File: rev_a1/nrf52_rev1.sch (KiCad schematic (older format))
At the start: 27 parts, among them P1 CONN_01X18, P2 CONN_01X18, P3 USB_OTG, U1 nRF52832, U2 CP2102, U3 LT1129CST-3.3, Y1 32K, Y2 32M

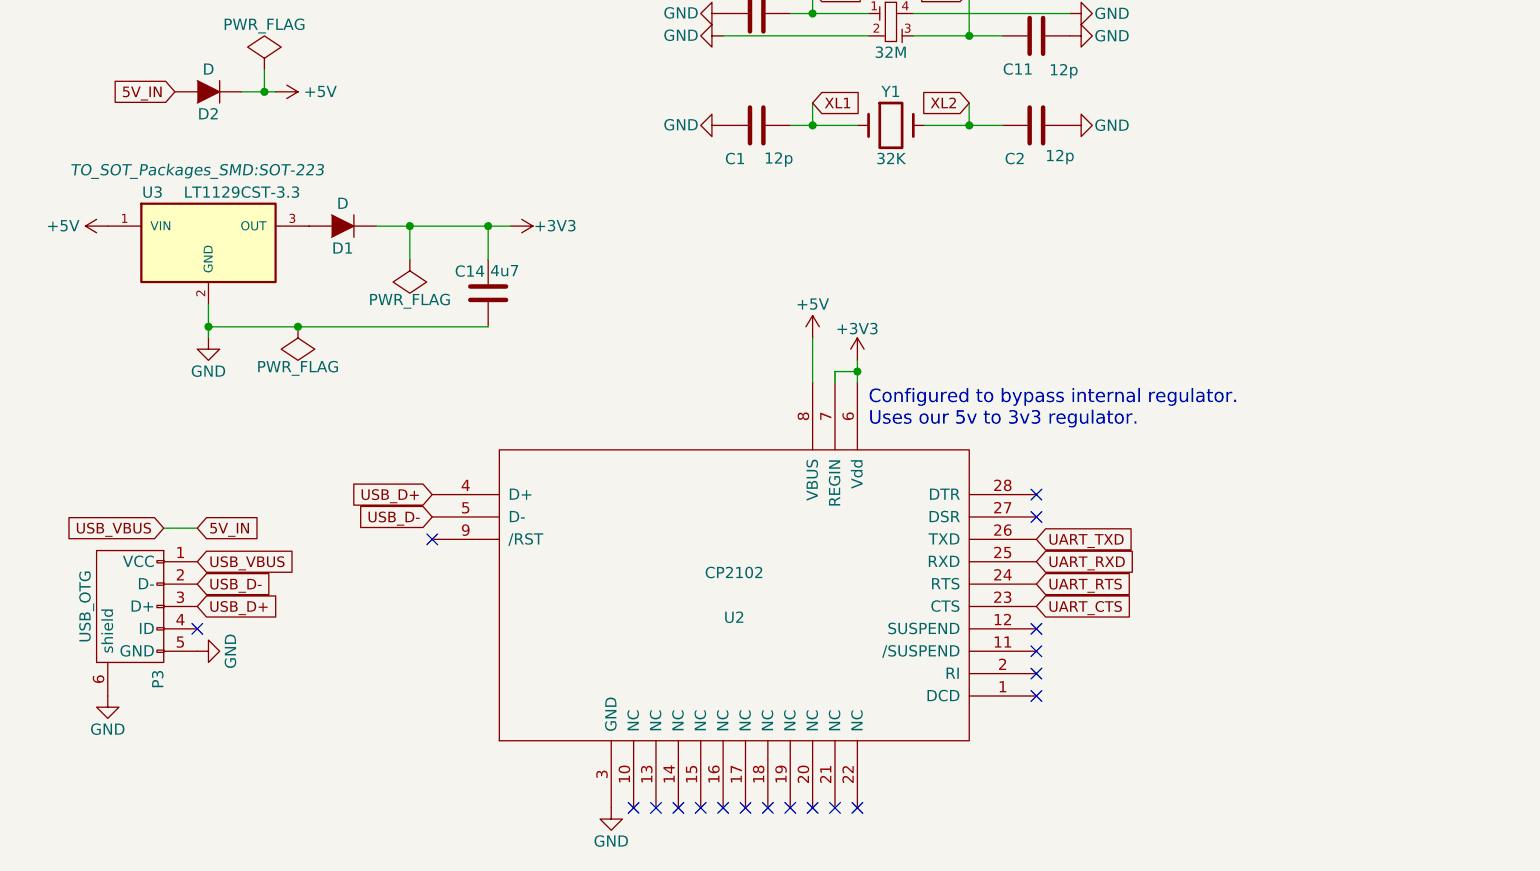
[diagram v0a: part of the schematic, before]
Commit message: wipwipwip
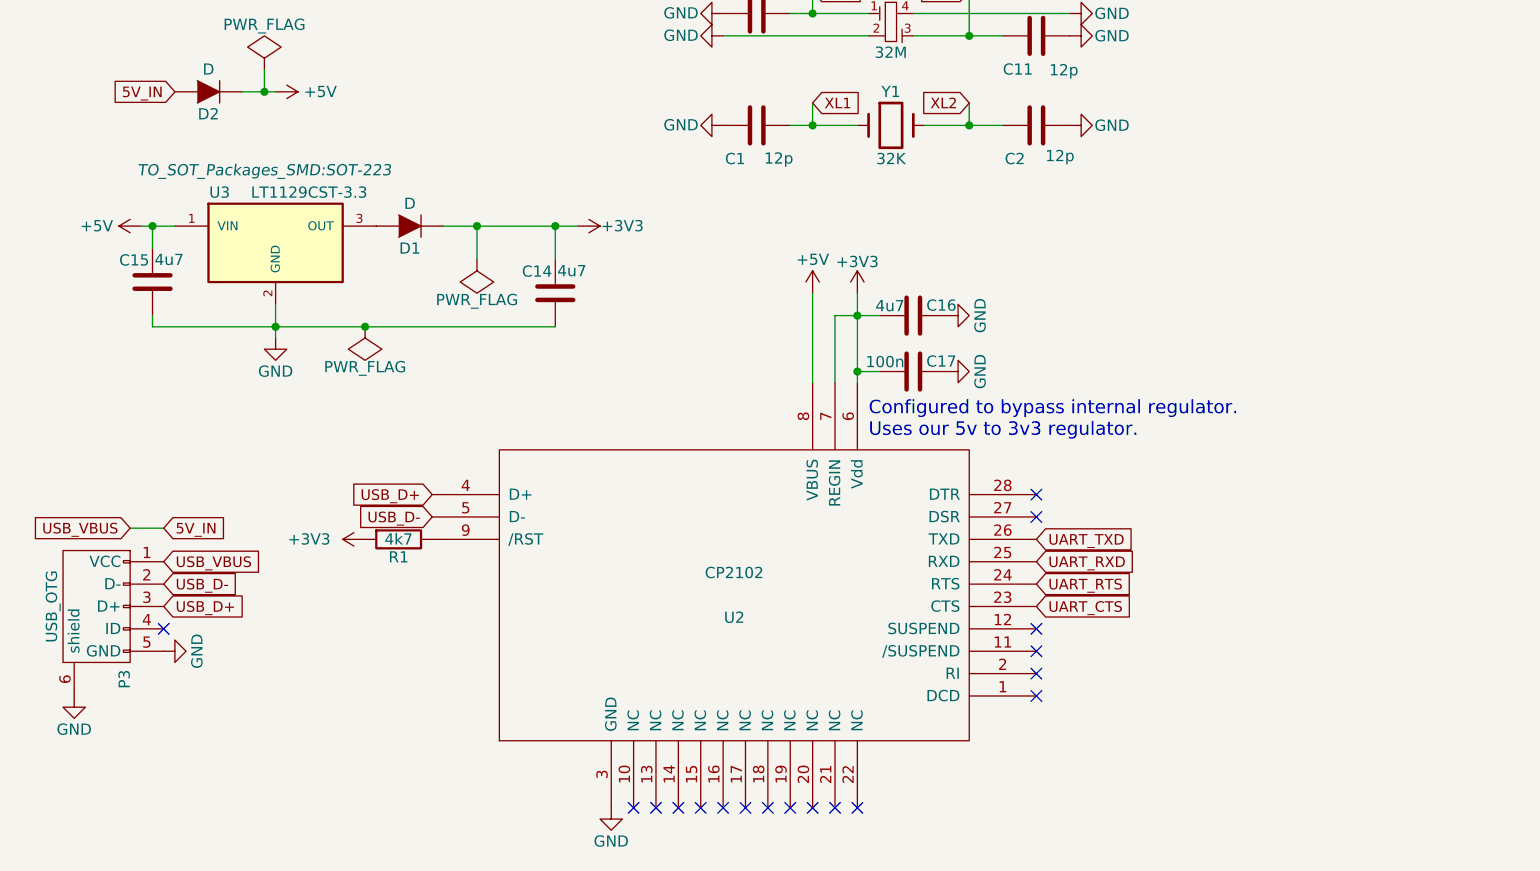
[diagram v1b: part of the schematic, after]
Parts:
- added C15, C16: 4u7, RuuviTag:0603_CAP, symbol C
- added C17: 100n, RuuviTag:0603_CAP, symbol C
- added R1: 4k7, symbol R
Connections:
- net +3V3: now also C16.2, C17.2, R1.2
- net +5V: now also C15.2
- net GND: now also C15.1, C16.1, C17.1
- net at U2.9 (/RST): now also R1.1
- no-connect marks 21 -> 20
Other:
- moved on the sheet: C14, D1, P3, U3

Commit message: wörk wörk
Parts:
- R1: footprint (none) -> RuuviTag:0603_RES
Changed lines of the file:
@@
 $EndDescr
 $Comp
-L GND #PWR28
+L GND #PWR01
 U 1 1 57587EFC
 P 6300 1300
-F 0 "#PWR28" H 6300 1050 50  0001 C CNN
+F 0 "#PWR01" H 6300 1050 50  0001 C CNN
 F 1 "GND" H 6300 1150 50  0000 C CNN
 F 2 "" H 6300 1300 50  0000 C CNN
@@
 $EndComp
 $Comp
-L GND #PWR9
+L GND #PWR02
 U 1 1 57588077
 P 2450 1000
-F 0 "#PWR9" H 2450 750 50  0001 C CNN
+F 0 "#PWR02" H 2450 750 50  0001 C CNN
 F 1 "GND" V 2449 812 50  0000 C CNN
 F 2 "" H 2450 1000 50  0000 C CNN
@@
 $EndComp
 $Comp
-L GND #PWR8
+L GND #PWR03
 U 1 1 57588655
 P 2450 900
-F 0 "#PWR8" H 2450 650 50  0001 C CNN
+F 0 "#PWR03" H 2450 650 50  0001 C CNN
 F 1 "GND" V 2449 712 50  0000 C CNN
 F 2 "" H 2450 900 50  0000 C CNN
@@
 $EndComp
 $Comp
-L GND #PWR7
+L GND #PWR04
 U 1 1 5758866C
 P 2450 800
-F 0 "#PWR7" H 2450 550 50  0001 C CNN
+F 0 "#PWR04" H 2450 550 50  0001 C CNN
 F 1 "GND" V 2449 612 50  0000 C CNN
 F 2 "" H 2450 800 50  0000 C CNN
@@
 $EndComp
 $Comp
-L GND #PWR12
+L GND #PWR05
 U 1 1 575887A0
 P 2450 1400
-F 0 "#PWR12" H 2450 1150 50  0001 C CNN
+F 0 "#PWR05" H 2450 1150 50  0001 C CNN
 F 1 "GND" V 2449 1212 50  0000 C CNN
 F 2 "" H 2450 1400 50  0000 C CNN
@@
 $EndComp
 $Comp
-L GND #PWR11
+L GND #PWR06
 U 1 1 575887B8
 P 2450 1300
-F 0 "#PWR11" H 2450 1050 50  0001 C CNN
+F 0 "#PWR06" H 2450 1050 50  0001 C CNN
 F 1 "GND" V 2449 1112 50  0000 C CNN
 F 2 "" H 2450 1300 50  0000 C CNN
@@
 $EndComp
 $Comp
-L GND #PWR10
+L GND #PWR07
 U 1 1 575887BE
 P 2450 1200
-F 0 "#PWR10" H 2450 950 50  0001 C CNN
+F 0 "#PWR07" H 2450 950 50  0001 C CNN
 F 1 "GND" V 2449 1012 50  0000 C CNN
 F 2 "" H 2450 1200 50  0000 C CNN
@@
 $EndComp
 $Comp
-L GND #PWR13
+L GND #PWR08
 U 1 1 57589680
 P 2450 1700
-F 0 "#PWR13" H 2450 1450 50  0001 C CNN
+F 0 "#PWR08" H 2450 1450 50  0001 C CNN
 F 1 "GND" V 2449 1512 50  0000 C CNN
 F 2 "" H 2450 1700 50  0000 C CNN
@@
 $EndComp
 $Comp
-L GND #PWR15
+L GND #PWR09
 U 1 1 57589C6C
 P 3050 3500
-F 0 "#PWR15" H 3050 3250 50  0001 C CNN
+F 0 "#PWR09" H 3050 3250 50  0001 C CNN
 F 1 "GND" V 3049 3312 50  0000 C CNN
 F 2 "" H 3050 3500 50  0000 C CNN
@@
 $EndComp
 $Comp
-L GND #PWR18
+L GND #PWR010
 U 1 1 57589C95
 P 3650 4000
-F 0 "#PWR18" H 3650 3750 50  0001 C CNN
+F 0 "#PWR010" H 3650 3750 50  0001 C CNN
 F 1 "GND" V 3649 3812 50  0000 C CNN
 F 2 "" H 3650 4000 50  0000 C CNN
@@
 $EndComp
 $Comp
-L GND #PWR19
+L GND #PWR011
 U 1 1 57589CBE
 P 3650 4100
-F 0 "#PWR19" H 3650 3850 50  0001 C CNN
+F 0 "#PWR011" H 3650 3850 50  0001 C CNN
 F 1 "GND" V 3649 3912 50  0000 C CNN
 F 2 "" H 3650 4100 50  0000 C CNN
@@
 $EndComp
 $Comp
-L GND #PWR26
+L GND #PWR012
 U 1 1 5758A08F
 P 5200 4100
-F 0 "#PWR26" H 5200 3850 50  0001 C CNN
+F 0 "#PWR012" H 5200 3850 50  0001 C CNN
 F 1 "GND" V 5199 3912 50  0000 C CNN
 F 2 "" H 5200 4100 50  0000 C CNN
@@
 $EndComp
 $Comp
-L GND #PWR25
+L GND #PWR013
 U 1 1 5758A0C1
 P 5200 4000
-F 0 "#PWR25" H 5200 3750 50  0001 C CNN
+F 0 "#PWR013" H 5200 3750 50  0001 C CNN
 F 1 "GND" V 5199 3812 50  0000 C CNN
 F 2 "" H 5200 4000 50  0000 C CNN
@@
 $EndComp
 $Comp
-L GND #PWR5
+L GND #PWR014
 U 1 1 5758E3CC
 P 1650 5450
-F 0 "#PWR5" H 1650 5200 50  0001 C CNN
+F 0 "#PWR014" H 1650 5200 50  0001 C CNN
 F 1 "GND" H 1650 5300 50  0000 C CNN
 F 2 "" H 1650 5450 50  0000 C CNN
@@
 $EndComp
 $Comp
-L PWR_FLAG #FLG2
+L PWR_FLAG #FLG015
 U 1 1 5758E406
 P 2050 5400
-F 0 "#FLG2" H 2050 5495 50  0001 C CNN
+F 0 "#FLG015" H 2050 5495 50  0001 C CNN
 F 1 "PWR_FLAG" H 2050 5580 50  0000 C CNN
 F 2 "" H 2050 5400 50  0000 C CNN
@@
 $EndComp
 $Comp
-L PWR_FLAG #FLG3
+L PWR_FLAG #FLG016
 U 1 1 5758E498
 P 2550 5100
-F 0 "#FLG3" H 2550 5195 50  0001 C CNN
+F 0 "#FLG016" H 2550 5195 50  0001 C CNN
 F 1 "PWR_FLAG" H 2550 5280 50  0000 C CNN
 F 2 "" H 2550 5100 50  0000 C CNN
@@
 $EndComp
 $Comp
-L GND #PWR29
+L GND #PWR017
 U 1 1 57592DA0
 P 7200 1100
-F 0 "#PWR29" H 7200 850 50  0001 C CNN
+F 0 "#PWR017" H 7200 850 50  0001 C CNN
 F 1 "GND" H 7200 950 50  0000 C CNN
 F 2 "" H 7200 1100 50  0000 C CNN
@@
 $EndComp
 $Comp
-L +3V3 #PWR14
+L +3V3 #PWR018
 U 1 1 57599355
 P 3000 4950
-F 0 "#PWR14" H 3000 4800 50  0001 C CNN
+F 0 "#PWR018" H 3000 4800 50  0001 C CNN
 F 1 "+3V3" V 3000 5150 50  0000 C CNN
 F 2 "" H 3000 4950 50  0000 C CNN
@@
 $EndComp
 $Comp
-L GND #PWR1
+L GND #PWR019
 U 1 1 57599CC0
 P 750 7050
-F 0 "#PWR1" H 750 6800 50  0001 C CNN
+F 0 "#PWR019" H 750 6800 50  0001 C CNN
 F 1 "GND" H 750 6900 50  0000 C CNN
 F 2 "" H 750 7050 50  0000 C CNN
@@
 $EndComp
 $Comp
-L GND #PWR3
+L GND #PWR020
 U 1 1 57599E62
 P 1150 6850
-F 0 "#PWR3" H 1150 6600 50  0001 C CNN
+F 0 "#PWR020" H 1150 6600 50  0001 C CNN
 F 1 "GND" H 1150 6700 50  0000 C CNN
 F 2 "" H 1150 6850 50  0000 C CNN
@@
 NoConn ~ 3550 7550
 $Comp
-L GND #PWR17
+L GND #PWR021
 U 1 1 5759B7C2
 P 3150 7550
-F 0 "#PWR17" H 3150 7300 50  0001 C CNN
+F 0 "#PWR021" H 3150 7300 50  0001 C CNN
 F 1 "GND" H 3150 7400 50  0000 C CNN
 F 2 "" H 3150 7550 50  0000 C CNN
@@
 $EndComp
 $Comp
-L +5V #PWR2
+L +5V #PWR022
 U 1 1 5759E11F
 P 1050 4950
-F 0 "#PWR2" H 1050 4800 50  0001 C CNN
+F 0 "#PWR022" H 1050 4800 50  0001 C CNN
 F 1 "+5V" V 1050 5150 50  0000 C CNN
 F 2 "" H 1050 4950 50  0000 C CNN
@@
 $EndComp
 $Comp
-L +3V3 #PWR22
+L +3V3 #PWR023
 U 1 1 5759E6E9
 P 4250 5250
-F 0 "#PWR22" H 4250 5100 50  0001 C CNN
+F 0 "#PWR023" H 4250 5100 50  0001 C CNN
 F 1 "+3V3" H 4250 5390 50  0000 C CNN
 F 2 "" H 4250 5250 50  0000 C CNN
@@
 5V_IN
 $Comp
-L +5V #PWR4
+L +5V #PWR024
 U 1 1 575C79F8
 P 1650 4350
-F 0 "#PWR4" H 1650 4200 50  0001 C CNN
+F 0 "#PWR024" H 1650 4200 50  0001 C CNN
 F 1 "+5V" V 1650 4550 50  0000 C CNN
 F 2 "" H 1650 4350 50  0000 C CNN
@@
 P0.31
 $Comp
-L +3V3 #PWR16
+L +3V3 #PWR025
 U 1 1 575CB207
 P 3150 700
-F 0 "#PWR16" H 3150 550 50  0001 C CNN
+F 0 "#PWR025" H 3150 550 50  0001 C CNN
 F 1 "+3V3" H 3150 850 50  0000 C CNN
 F 2 "" H 3150 700 50  0000 C CNN
@@
 $EndComp
 $Comp
-L GND #PWR20
+L GND #PWR026
 U 1 1 575D0E9A
 P 3650 4500
-F 0 "#PWR20" H 3650 4250 50  0001 C CNN
+F 0 "#PWR026" H 3650 4250 50  0001 C CNN
 F 1 "GND" V 3649 4312 50  0000 C CNN
 F 2 "" H 3650 4500 50  0000 C CNN
@@
 $EndComp
 $Comp
-L GND #PWR27
+L GND #PWR027
 U 1 1 575D0EA0
 P 5200 4500
-F 0 "#PWR27" H 5200 4250 50  0001 C CNN
+F 0 "#PWR027" H 5200 4250 50  0001 C CNN
 F 1 "GND" V 5199 4312 50  0000 C CNN
 F 2 "" H 5200 4500 50  0000 C CNN
@@
 SWDCLK
 $Comp
-L +5V #PWR21
+L +5V #PWR028
 U 1 1 575DB331
 P 4050 5250
-F 0 "#PWR21" H 4050 5100 50  0001 C CNN
+F 0 "#PWR028" H 4050 5100 50  0001 C CNN
 F 1 "+5V" H 4050 5400 50  0000 C CNN
 F 2 "" H 4050 5250 50  0000 C CNN
@@
 $EndComp
 $Comp
-L PWR_FLAG #FLG1
+L PWR_FLAG #FLG029
 U 1 1 575DB491
 P 1600 4250
-F 0 "#FLG1" H 1600 4345 50  0001 C CNN
+F 0 "#FLG029" H 1600 4345 50  0001 C CNN
 F 1 "PWR_FLAG" H 1600 4450 50  0000 C CNN
 F 2 "" H 1600 4250 50  0000 C CNN
@@
 SWO
 $Comp
-L GND #PWR31
+L GND #PWR030
 U 1 1 575DC1F5
 P 9150 6250
-F 0 "#PWR31" H 9150 6000 50  0001 C CNN
+F 0 "#PWR030" H 9150 6000 50  0001 C CNN
 F 1 "GND" V 9150 6050 50  0000 C CNN
 F 2 "" H 9150 6250 50  0000 C CNN
@@
 $EndComp
 $Comp
-L +3V3 #PWR30
+L +3V3 #PWR031
 U 1 1 575DC6AD
 P 9150 6150
-F 0 "#PWR30" H 9150 6000 50  0001 C CNN
+F 0 "#PWR031" H 9150 6000 50  0001 C CNN
 F 1 "+3V3" V 9151 6378 50  0000 C CNN
 F 2 "" H 9150 6150 50  0000 C CNN
@@
 $EndComp
 $Comp
-L GND #PWR32
+L GND #PWR032
 U 1 1 575DC996
 P 9850 4550
-F 0 "#PWR32" H 9850 4300 50  0001 C CNN
+F 0 "#PWR032" H 9850 4300 50  0001 C CNN
 F 1 "GND" V 9850 4350 50  0000 C CNN
 F 2 "" H 9850 4550 50  0000 C CNN
@@
 $EndComp
 $Comp
-L +3V3 #PWR34
+L +3V3 #PWR033
 U 1 1 575DCAE2
 P 9850 4850
-F 0 "#PWR34" H 9850 4700 50  0001 C CNN
+F 0 "#PWR033" H 9850 4700 50  0001 C CNN
 F 1 "+3V3" V 9849 5073 50  0000 C CNN
 F 2 "" H 9850 4850 50  0000 C CNN
@@
 $EndComp
 $Comp
-L GND #PWR33
+L GND #PWR034
 U 1 1 575DCBF4
 P 9850 4750
-F 0 "#PWR33" H 9850 4500 50  0001 C CNN
+F 0 "#PWR034" H 9850 4500 50  0001 C CNN
 F 1 "GND" V 9850 4550 50  0000 C CNN
 F 2 "" H 9850 4750 50  0000 C CNN
@@
 F 0 "R1" V 2280 6350 50  0000 C CNN
 F 1 "4k7" V 2200 6350 50  0000 C CNN
-F 2 "" V 2130 6350 50  0000 C CNN
+F 2 "RuuviTag:0603_RES" V 2130 6350 50  0001 C CNN
 F 3 "" H 2200 6350 50  0000 C CNN
 	1    2200 6350
@@
 $EndComp
 $Comp
-L +3V3 #PWR6
+L +3V3 #PWR035
 U 1 1 575DCF2A
 P 2050 6350
-F 0 "#PWR6" H 2050 6200 50  0001 C CNN
+F 0 "#PWR035" H 2050 6200 50  0001 C CNN
 F 1 "+3V3" V 2050 6600 50  0000 C CNN
 F 2 "" H 2050 6350 50  0000 C CNN
@@
 $EndComp
 $Comp
-L GND #PWR24
+L GND #PWR036
 U 1 1 575DD677
 P 4650 5600
-F 0 "#PWR24" H 4650 5350 50  0001 C CNN
+F 0 "#PWR036" H 4650 5350 50  0001 C CNN
 F 1 "GND" H 4650 5450 50  0000 C CNN
 F 2 "" H 4650 5600 50  0000 C CNN
@@
 $EndComp
 $Comp
-L GND #PWR23
+L GND #PWR037
 U 1 1 575DED7D
 P 4650 5350
-F 0 "#PWR23" H 4650 5100 50  0001 C CNN
+F 0 "#PWR037" H 4650 5100 50  0001 C CNN
 F 1 "GND" H 4650 5200 50  0000 C CNN
 F 2 "" H 4650 5350 50  0000 C CNN
@@
 Wire Wire Line
 	3150 700  3150 1000
-Wire Wire Line
-	4250 5250 4250 5650
-Wire Wire Line
-	4250 5600 4350 5600
-Wire Wire Line
-	4150 5650 4150 5350
-Wire Wire Line
-	4150 5350 4350 5350
-Connection ~ 4250 5350
-Connection ~ 4250 5600
 $Comp
 L C C15
@@
 Wire Wire Line
 	1100 5400 1100 5350
+Connection ~ 4250 5600
+Wire Wire Line
+	4250 5600 4350 5600
+Connection ~ 4250 5350
+Wire Wire Line
+	4150 5350 4350 5350
+Wire Wire Line
+	4150 5650 4150 5350
+Wire Wire Line
+	4250 5250 4250 5650
 $EndSCHEMATC
